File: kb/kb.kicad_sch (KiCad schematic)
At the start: 109 parts, among them J1 Conn_01x04_MountingPin, SW1 SW_Push, SW10 SW_Push, SW11 SW_Push, SW12 SW_Push, SW13 SW_Push, SW14 SW_Push, SW15 SW_Push, SW16 SW_Push, SW17 SW_Push, SW18 SW_Push, SW19 SW_Push, SW2 SW_Push, SW20 SW_Push, SW21 SW_Push, SW22 SW_Push, SW23 SW_Push, SW24 SW_Push, SW25 SW_Push, SW26 SW_Push, SW27 SW_Push, SW28 SW_Push, SW29 SW_Push, SW3 SW_Push, SW30 SW_Push, SW31 SW_Push, SW32 SW_Push, SW33 SW_Push, SW34 SW_Push, SW35 SW_Push, SW36 SW_Push, SW37 SW_Push, SW38 SW_Push, SW39 SW_Push, SW4 SW_Push, SW40 SW_Push, SW41 SW_Push, SW42 SW_Push, SW43 SW_Push, SW44 SW_Push, SW45 SW_Push, SW46 SW_Push, SW48 SW_Push, SW5 SW_Push, SW6 SW_Push, SW7 SW_Push, SW8 SW_Push, SW9 SW_Push, U1 USBLC6-2SC6, U2 STM32G474CETx, U4 XC6206PxxxMR

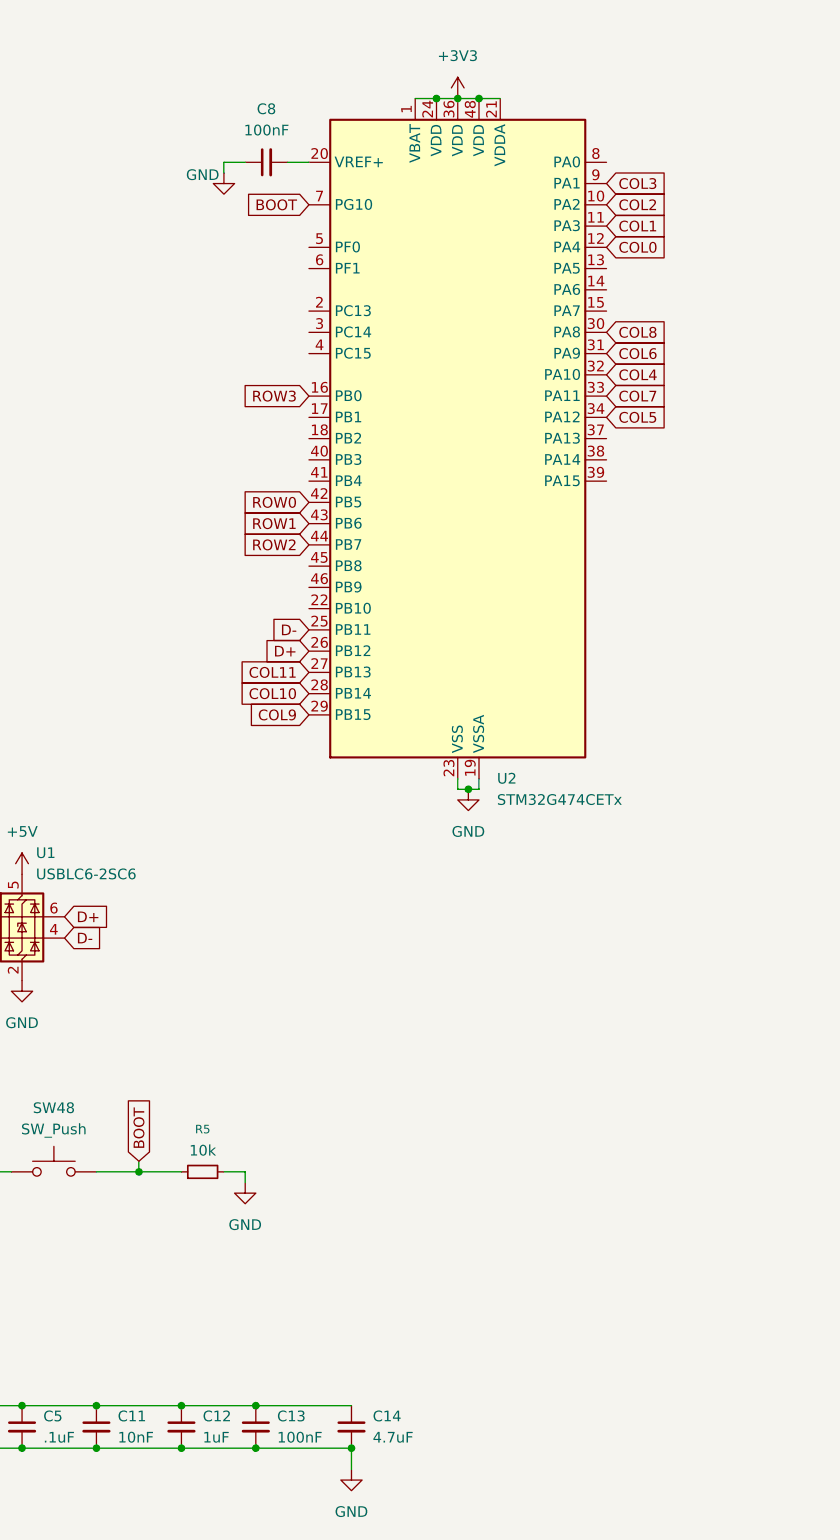
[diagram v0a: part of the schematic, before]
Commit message: Fixed Board Side
Fixed Side of board
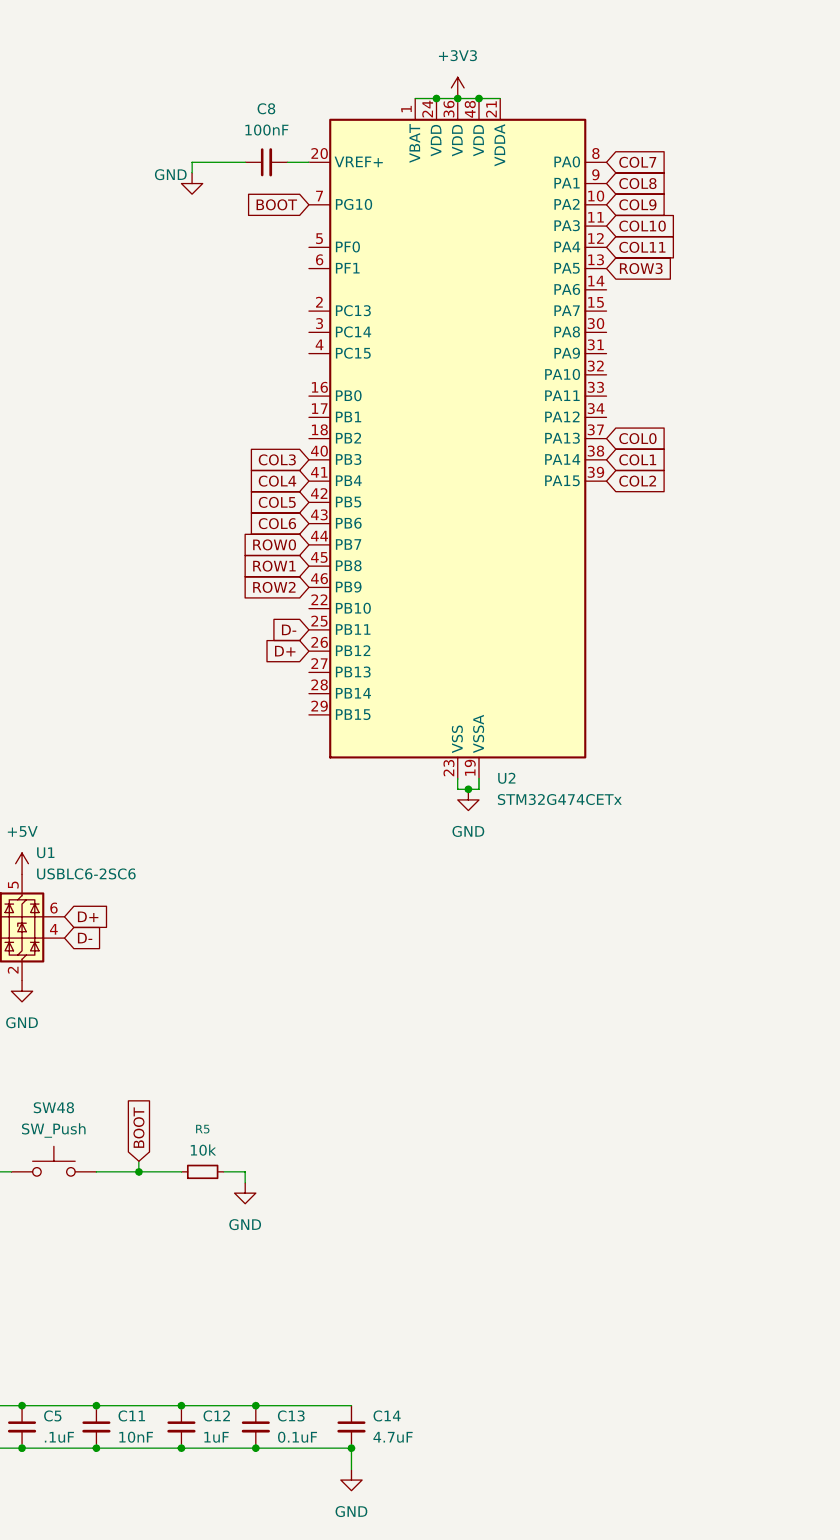
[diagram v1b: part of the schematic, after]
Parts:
- C13: value 100nF -> 0.1uF
- D1, D10, D11, D12, D13, D14, D15, D16, D17, D18, D19, D2, D20, D21, D22, D23, D24, D25, D26, D27, D28, D29, D3, D30, D31, D32, D33, D34, D35, D36, D37, D38, D39, D4, D40, D41, D42, D43, D44, D45, D46, D5, D6, D7, D8, D9: footprint Diode_SMD:D_0201_0603Metric -> Diode_SMD:D_0805_2012Metric
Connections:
- net COL0: now also U2.37 (PA13); no longer U2.12 (PA4)
- net COL1: now also U2.38 (PA14); no longer U2.11 (PA3)
- net COL10: now also U2.11 (PA3); no longer U2.28 (PB14)
- net COL11: now also U2.12 (PA4); no longer U2.27 (PB13)
- net COL2: now also U2.39 (PA15); no longer U2.10 (PA2)
- net COL3: now also U2.40 (PB3); no longer U2.9 (PA1)
- net COL4: now also U2.41 (PB4); no longer U2.32 (PA10)
- net COL5: now also U2.42 (PB5); no longer U2.34 (PA12)
- net COL6: now also U2.43 (PB6); no longer U2.31 (PA9)
- net COL7: now also U2.8 (PA0); no longer U2.33 (PA11)
- net COL8: now also U2.9 (PA1); no longer U2.30 (PA8)
- net COL9: now also U2.10 (PA2); no longer U2.29 (PB15)
- net ROW0: now also U2.44 (PB7); no longer U2.42 (PB5)
- net ROW1: now also U2.45 (PB8); no longer U2.43 (PB6)
- net ROW2: now also U2.46 (PB9); no longer U2.44 (PB7)
- net ROW3: now also U2.13 (PA5); no longer U2.16 (PB0)
